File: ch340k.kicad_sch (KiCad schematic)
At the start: 8 parts, among them J1 USB_B_Mini, J2 Conn_01x06_Male, U1 CH340K

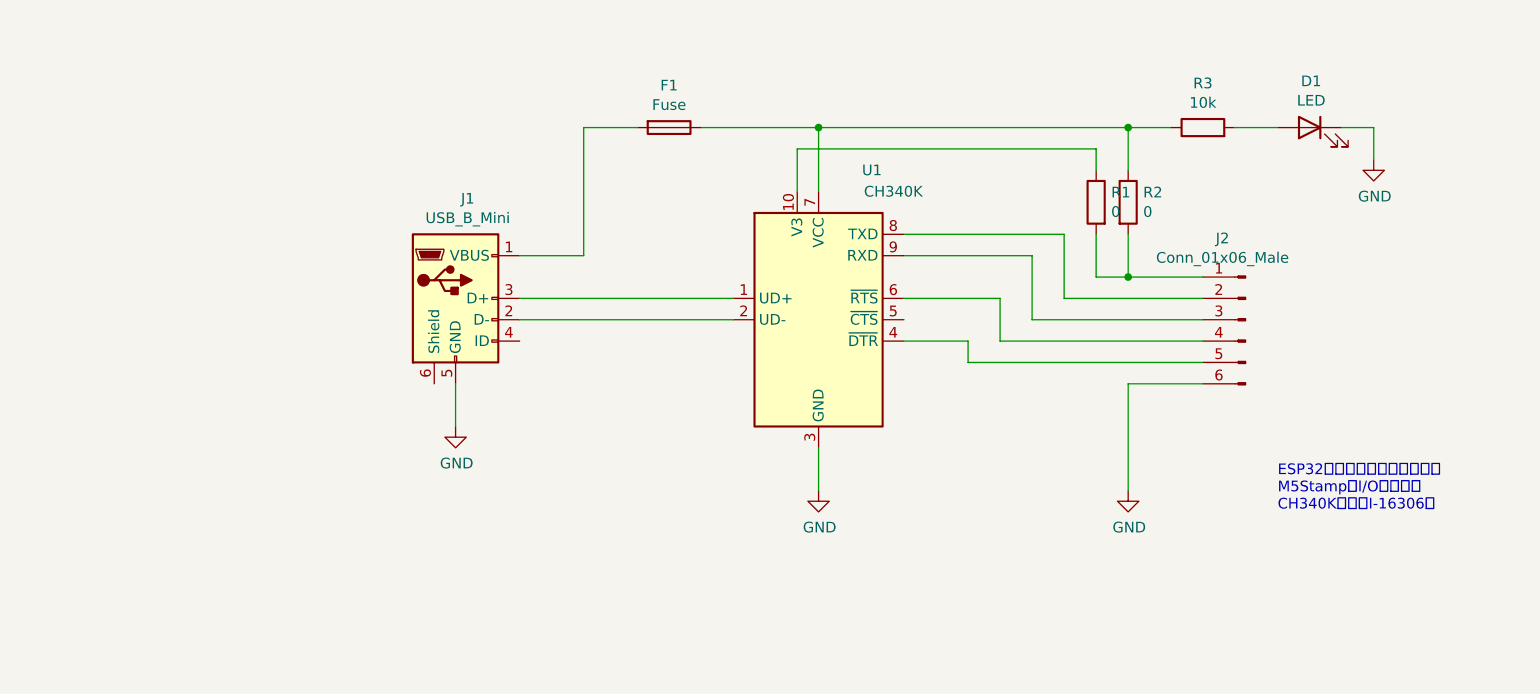
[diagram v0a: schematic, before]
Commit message: CW Interface prototype
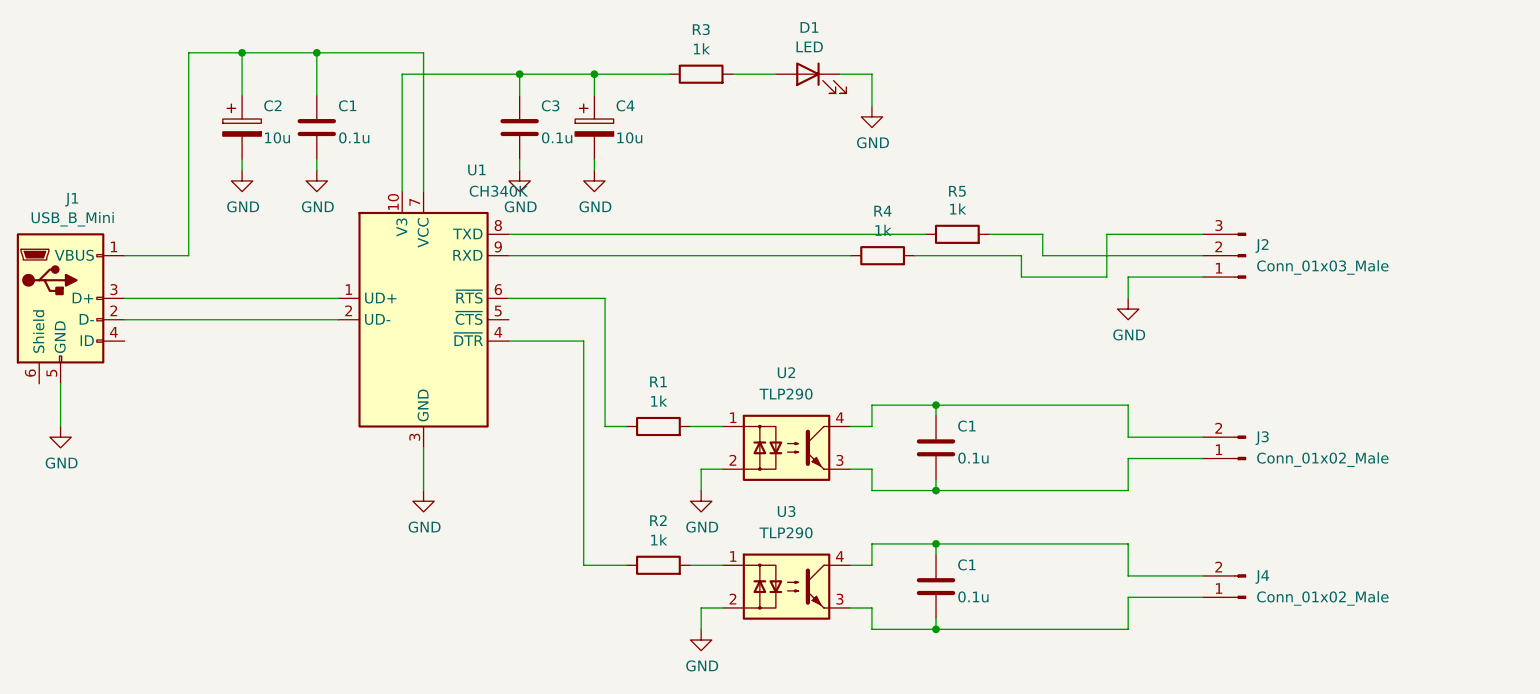
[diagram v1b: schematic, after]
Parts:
- removed F1: Fuse, digikey-footprints:0603, symbol Device:Fuse
- removed J2: Conn_01x06_Male, Connector_PinHeader_2.54mm:PinHeader_1x06_P2.54mm_Vertical, symbol Connector:Conn_01x06_Male
- added C1 (x3), C3: 0.1u, UserLib:0603, symbol Device:C
- added C2, C4: 10u, Capacitor_THT:CP_Radial_D5.0mm_P2.00mm, symbol Device:C_Polarized
- added J2: Conn_01x03_Male, Connector_PinHeader_2.54mm:PinHeader_1x03_P2.54mm_Vertical, symbol Connector:Conn_01x03_Male
- added J3, J4: Conn_01x02_Male, Connector_PinHeader_2.54mm:PinHeader_1x02_P2.54mm_Vertical, symbol Connector:Conn_01x02_Male
- added R4, R5: 1k, UserLib:0603, symbol Device:R
- added U2, U3: TLP290, Package_SO:SOP-4_4.4x2.6mm_P1.27mm, symbol Isolator:TLP290
- D1: footprint digikey-footprints:LED_2-SMD_No_Lead_1.7x0.8mm -> UserLib:0603
- R1, R2: value 0 -> 1k; footprint digikey-footprints:0603 -> UserLib:0603
- R3: value 10k -> 1k; footprint digikey-footprints:0603 -> UserLib:0603
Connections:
- net GND: now also C1.2, C2.2, C3.2, C4.2, J2.1 (Pin_1), U2.2, U3.2
- net at R1.2: now also U2.1; no longer R2.2
- net at U1.8 (TXD): now also R5.1
- net at U1.9 (RXD): now also R4.1
- net at U1.6 (~{RTS}): now also R1.1
- net at U1.4 (~{DTR}): now also R2.1
- net at U1.10 (V3): now also R3.1, C3.1, C4.1; no longer R1.1
- net at J1.1 (VBUS): now also U1.7 (VCC), C1.1, C2.1
- new net: C1.2, J3.1 (Pin_1), U2.3
- new net: C1.1, J3.2 (Pin_2), U2.4
- new net: J2.2 (Pin_2), R5.2
- new net: R2.2, U3.1
- new net: C1.2, J4.1 (Pin_1), U3.3
- new net: C1.1, J4.2 (Pin_2), U3.4
- new net: J2.3 (Pin_3), R4.2
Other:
- note removed: "ESP32プログラムダウンローダ M5StampのI/O配列相当 CH340K（秋月I-16306）"
- moved on the sheet: D1, J1, R3, U1
